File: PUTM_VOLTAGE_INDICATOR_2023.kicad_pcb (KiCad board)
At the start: 2 copper layers, 35 parts, among them IC1 LM211DT, J1 HV+, J2 HV-, Q1 TK3P80E,RQ, U1 LT8316EFE

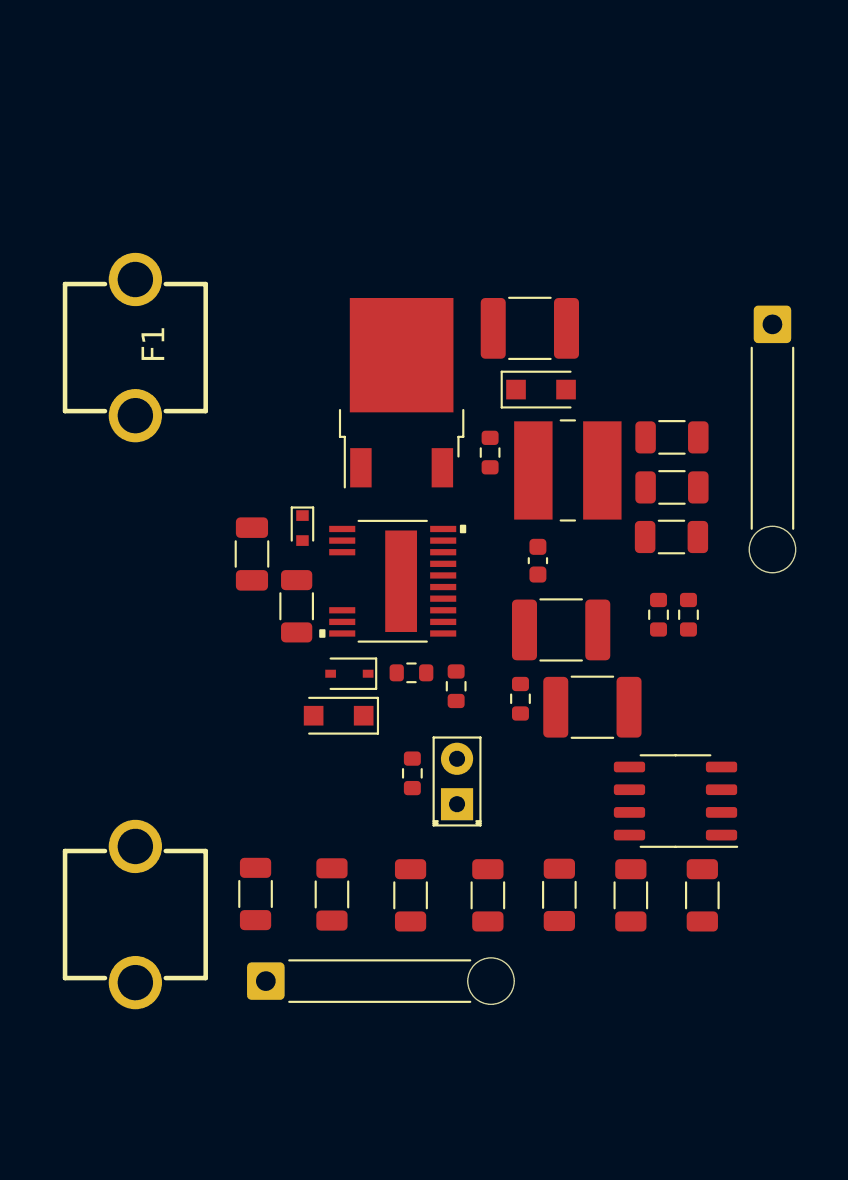
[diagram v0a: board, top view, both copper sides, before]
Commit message: Update PUTM_VOLTAGE_INDICATOR_2023.kicad_pcb
pcb update
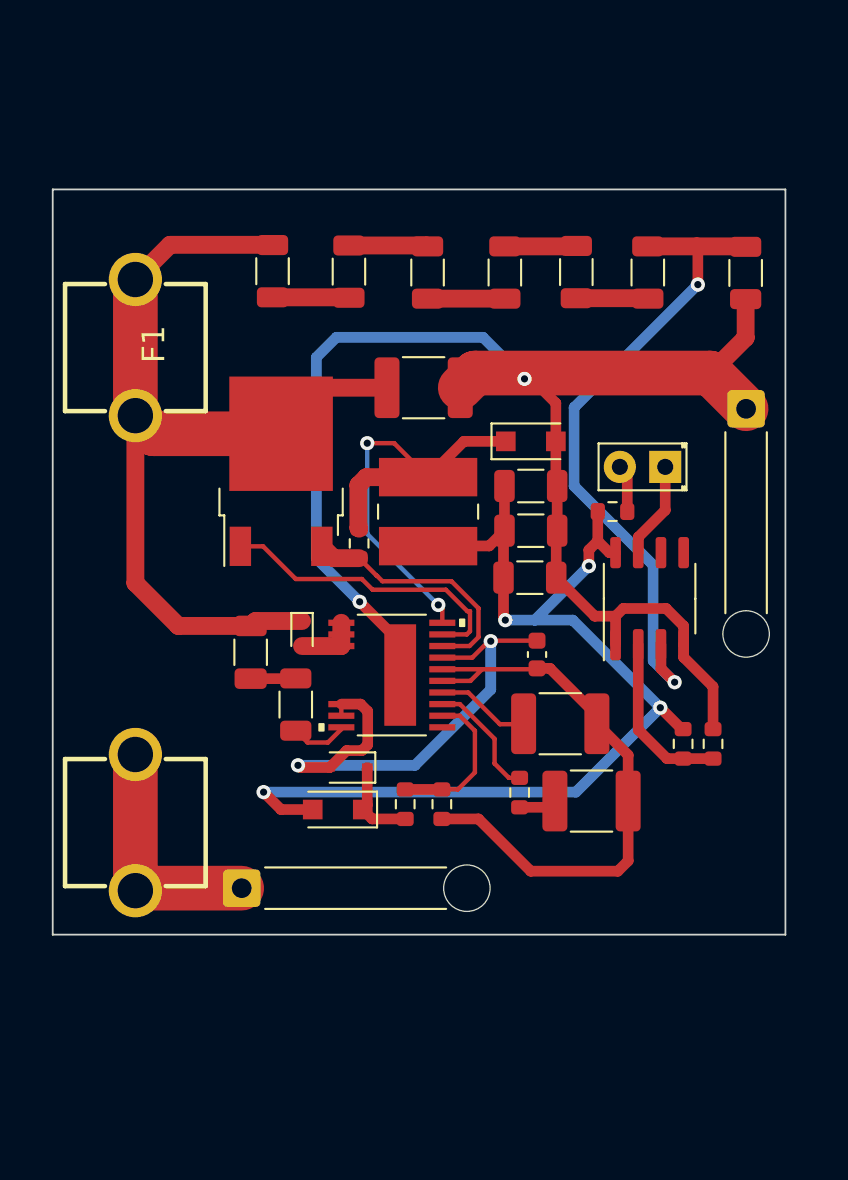
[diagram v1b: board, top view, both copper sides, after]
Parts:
- moved R7 34.9 mm to (131.8, 98.0)
- moved R3 34.9 mm to (114.0, 98.0)
- moved R4 34.9 mm to (118.3, 98.0)
- moved R5 34.9 mm to (122.3, 97.9)
- moved R6 34.9 mm to (126.3, 98.0)
- moved R1 34.9 mm to (105.3, 97.9)
- moved R2 34.9 mm to (109.6, 97.9)
- moved D1 22.2 mm to (127.3, 108.8), turned to 180 degrees
- moved R14 18.4 mm to (124.3, 111.3), turned to 0 degrees
- moved IC1 11.4 mm to (126.4, 116.2), turned to 90 degrees
- moved R19 8.92 mm to (110.1, 113.1)
- moved C8 8.35 mm to (119.8, 109.9)
- moved C7 8.26 mm to (119.8, 112.4)
- moved C6 8.25 mm to (119.7, 115.0)
- moved L1 8.15 mm to (114.0, 111.3), turned to -90 degrees
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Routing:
- net GND: track 0.00 -> 87.5 mm, vias 0 -> 2
- net Net-(C1-Pad2): track 0.00 -> 62.1 mm, vias 0 -> 2
- net +12V: track 0.00 -> 60.8 mm, vias 0 -> 4
- net +VDC: track 0.00 -> 51.6 mm
- net Net-(IC1-Pad3): track 0.00 -> 37.5 mm, vias 0 -> 2
- net Net-(C1-Pad1): track 0.00 -> 29.7 mm, vias 0 -> 2
- net Net-(Q1-Pad1): track 0.00 -> 17.2 mm
- net Net-(Q1-Pad3): track 0.00 -> 14.0 mm
- net Net-(F1-Pad2): track 0.00 -> 13.6 mm
- net Net-(IC1-Pad2): track 0.00 -> 9.62 mm
- net Net-(R15-Pad1): track 0.00 -> 8.80 mm
- net Net-(R17-Pad2): track 0.00 -> 6.84 mm
- net Net-(D1-Pad1): track 0.00 -> 5.43 mm
- net Net-(C3-Pad1): track 0.00 -> 5.30 mm
- net Net-(D2-Pad1): track 0.00 -> 5.05 mm
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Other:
- board outline added: 41 x 41.7 mm

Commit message: pcb update
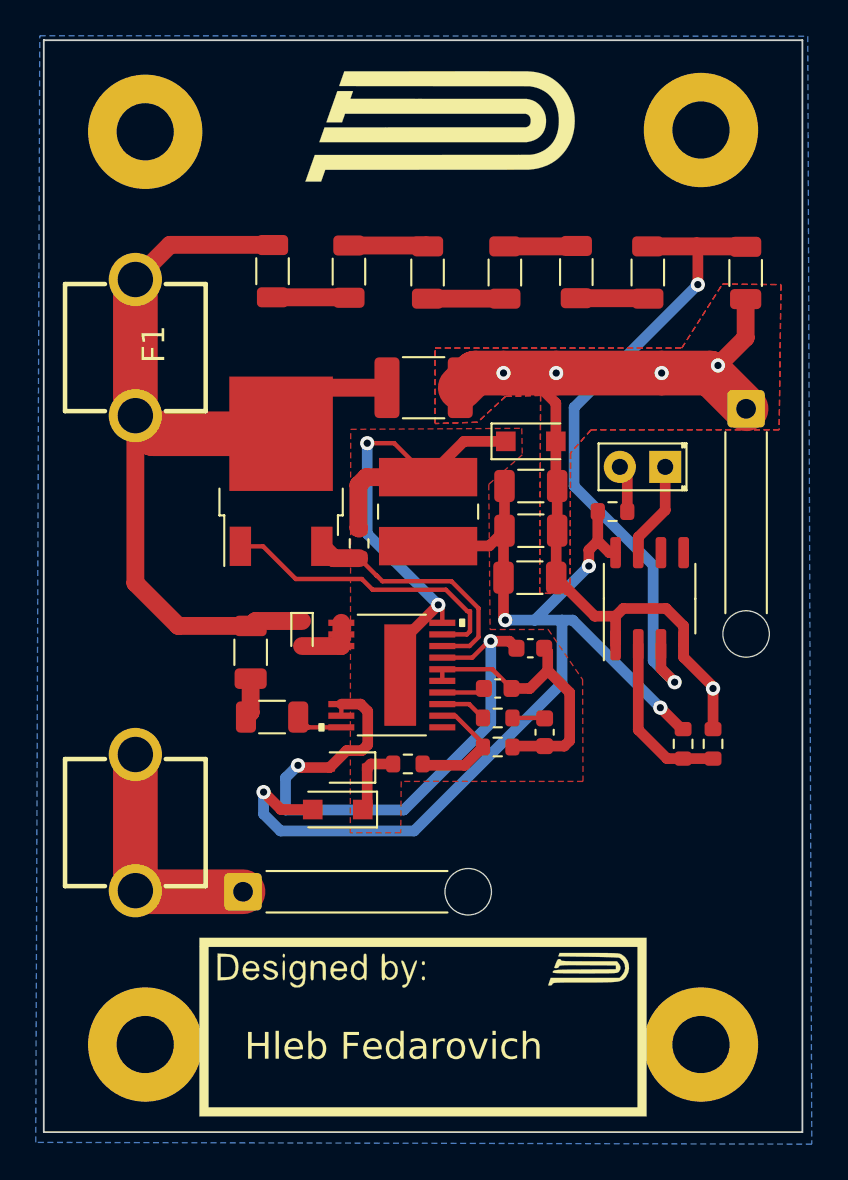
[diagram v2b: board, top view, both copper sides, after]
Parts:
- added ?: , , F.Cu at (129.3, 140.5)
- added ?: , , F.Cu at (97.8, 90.1)
- added ?: , , F.Cu at (129.2, 90.0)
- added ?: , , F.Cu at (99.0, 141.8)
- added G***: LOGO, SignatureBox25mm, F.Cu at (113.7, 140.2)
- added G***: LOGO, PUTM_LOGO_18mm, F.Cu at (114.2, 89.6)
- C2, C3: footprint Capacitor_SMD:C_1812_4532Metric -> Capacitor_SMD:C_0603_1608Metric
- moved C2 4.66 mm to (120.5, 123.7), turned to -90 degrees
- moved R16 4.47 mm to (117.9, 124.5), turned to 180 degrees
- moved R17 4.35 mm to (117.9, 122.9), turned to 180 degrees
- moved C3 4.02 mm to (117.9, 121.2)
- moved R15 2.25 mm to (112.9, 125.5), turned to 180 degrees
- moved R18 1.50 mm to (105.3, 122.8), turned to 0 degrees
- moved C1 0.51 mm to (119.7, 119.0), turned to 0 degrees
- moved J1 0.21 mm to (103.7, 132.6)
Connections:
- U1 pad EPAD: GND -> Net-(C1-Pad2)
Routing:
- net GND: track 87.5 -> 54.7 mm, vias 2 -> 5
- net Net-(C1-Pad2): track 62.1 -> 52.4 mm
- net Net-(C1-Pad1): track 29.7 -> 34.2 mm
- net Net-(R17-Pad2): track 6.84 -> 2.60 mm
- net Net-(C3-Pad1): track 5.30 -> 2.42 mm
- net Net-(R15-Pad1): track 8.80 -> 6.95 mm
- net +12V: track 60.8 -> 62.1 mm
- net Net-(D2-Pad1): track 5.05 -> 3.99 mm
- net Net-(R18-Pad2): track 3.24 -> 2.65 mm
- added copper zone on B.Cu, net GND
- added copper zone on F.Cu, net GND
- added copper zone on F.Cu, net Net-(C1-Pad2)
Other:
- board size 41 x 41.7 mm -> 42.4 x 61.1 mm
